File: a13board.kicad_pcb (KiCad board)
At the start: 4 copper layers, 99.8 x 45.7 mm, 147 parts, among them U1 H27UBG8T2A/TSOP48, U2 A13, U3 H5TQ2G43CFR, U4 H5TQ2G43CFR, U5 OLIMEX_IC_AXP209, U6 SY8008BAAC, U7 SY8008BAAC

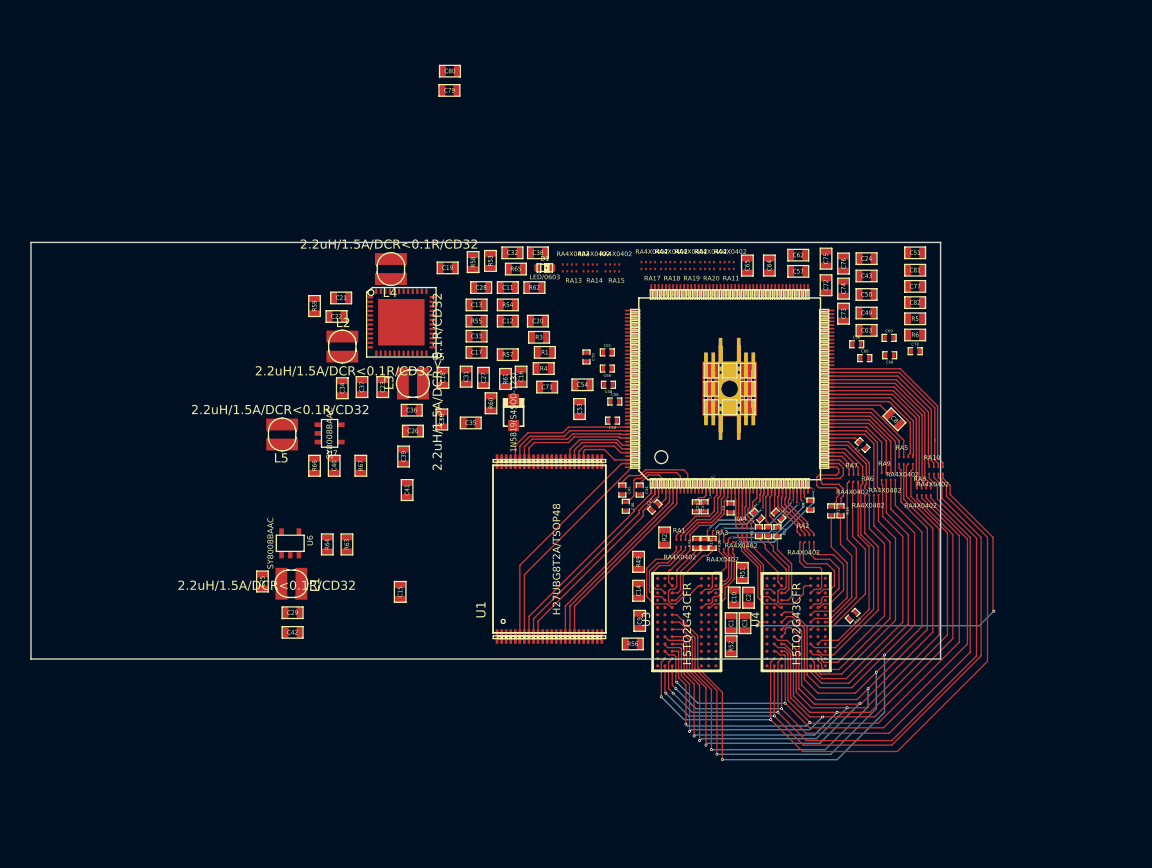
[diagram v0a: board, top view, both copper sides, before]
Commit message: still routing ddr3
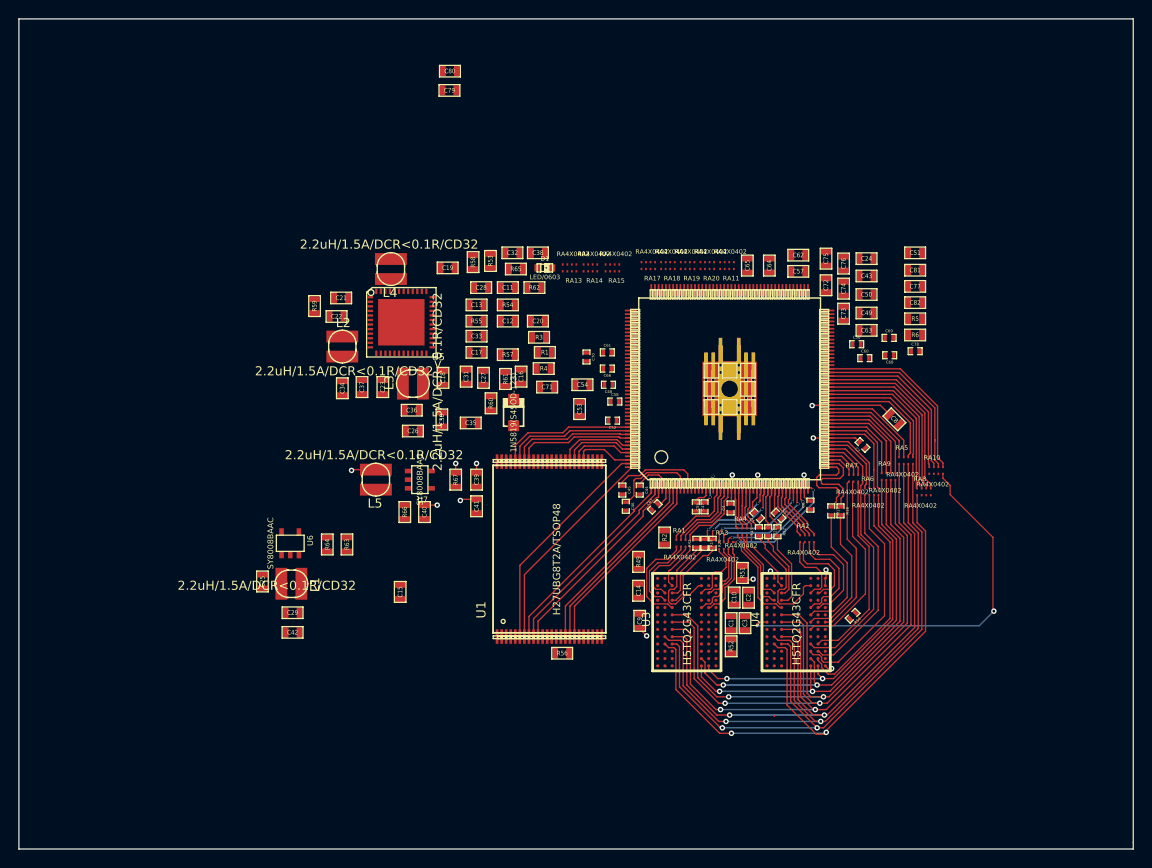
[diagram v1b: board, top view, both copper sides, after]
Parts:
- moved L5 11.4 mm to (74.7, 101.0)
- moved C40 11.1 mm to (80.0, 104.5)
- moved R66 11.1 mm to (77.9, 104.5)
- moved U7 11.1 mm to (79.5, 101.0)
- moved R67 10.5 mm to (83.4, 101.0)
- moved C39 8.39 mm to (85.7, 101.0)
- moved C41 7.82 mm to (85.7, 103.9)
- moved R56 7.81 mm to (95.1, 120.0)
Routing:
- net /DRAM/DDR3_A7: track 76.4 -> 0.00 mm, vias 2 -> 0
- net /DRAM/DDR3_A9: track 71.7 -> 0.00 mm, vias 2 -> 0
- net /DRAM/DDR3_RST: track 71.7 -> 0.14 mm, vias 2 -> 0
- net /DRAM/DDR3_A2: track 70.2 -> 0.00 mm, vias 2 -> 0
- net /DRAM/DDR3_A5: track 67.0 -> 0.00 mm, vias 2 -> 0
- net /DRAM/DDR3_A13: track 64.4 -> 0.00 mm, vias 2 -> 0
- net VMEM: track 17.4 -> 75.6 mm, vias 0 -> 14
- net /DRAM/DDR3_RAS: track 85.8 -> 64.9 mm
- net /DRAM/DDR3_CAS: track 83.3 -> 65.0 mm
- net /DRAM/DDR3_WE: track 82.8 -> 66.6 mm
- net /DRAM/DDR3_A11: track 30.7 -> 45.5 mm, vias 0 -> 2
- net /DRAM/DDR3_A14: track 31.4 -> 45.9 mm, vias 0 -> 2
- net /DRAM/DDR3_A8: track 26.2 -> 39.6 mm, vias 0 -> 2
- net /DRAM/DDR3_BA2: track 80.3 -> 67.5 mm
- net /DRAM/DDR3_BA0: track 79.3 -> 69.7 mm
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- added copper zone on Inner1.Cu, net VMEM
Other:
- board size 99.8 x 45.7 mm -> 122.3 x 91.1 mm
- net class Default: via_dia 0.31 -> 0.6
- net class bga: via_dia 0.31 -> 0.6
- net class power added: clearance 2, trace_width 0.2, via_dia 0.6, via_drill 0.3
- net class powersm added: clearance 0.15, trace_width 0.2, via_dia 0.6, via_drill 0.3
- rule via_min_size: 0.3 -> 0.6
